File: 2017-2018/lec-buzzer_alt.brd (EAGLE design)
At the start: 160 x 100 mm, 26 parts, among them K1 SKQGADE010, K2 SKQGADE010, K3 SKQGADE010, U1 ATMEGA328P-MUR

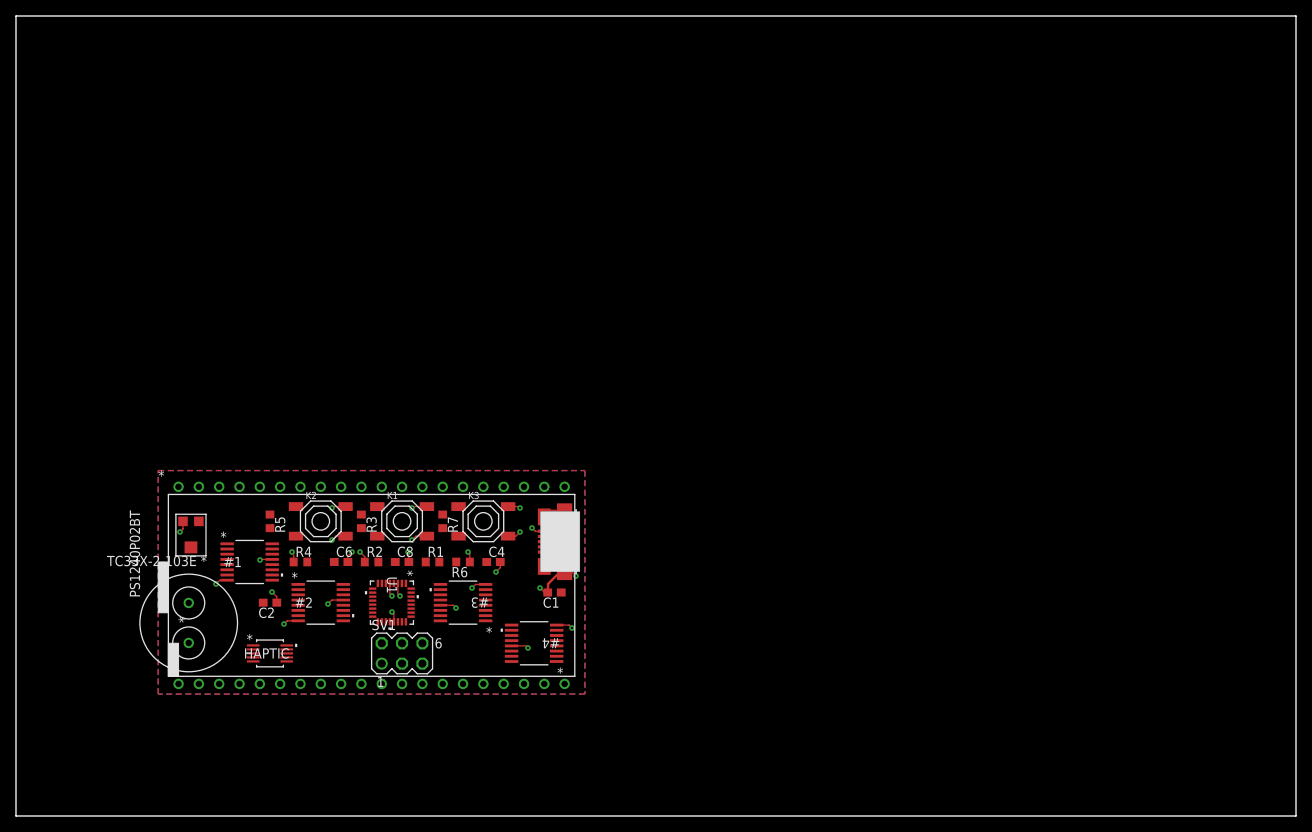
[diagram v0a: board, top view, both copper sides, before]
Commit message: 3 Button Board completed
LCD flipped, slight changes in shifter, Buzzer and SPI location
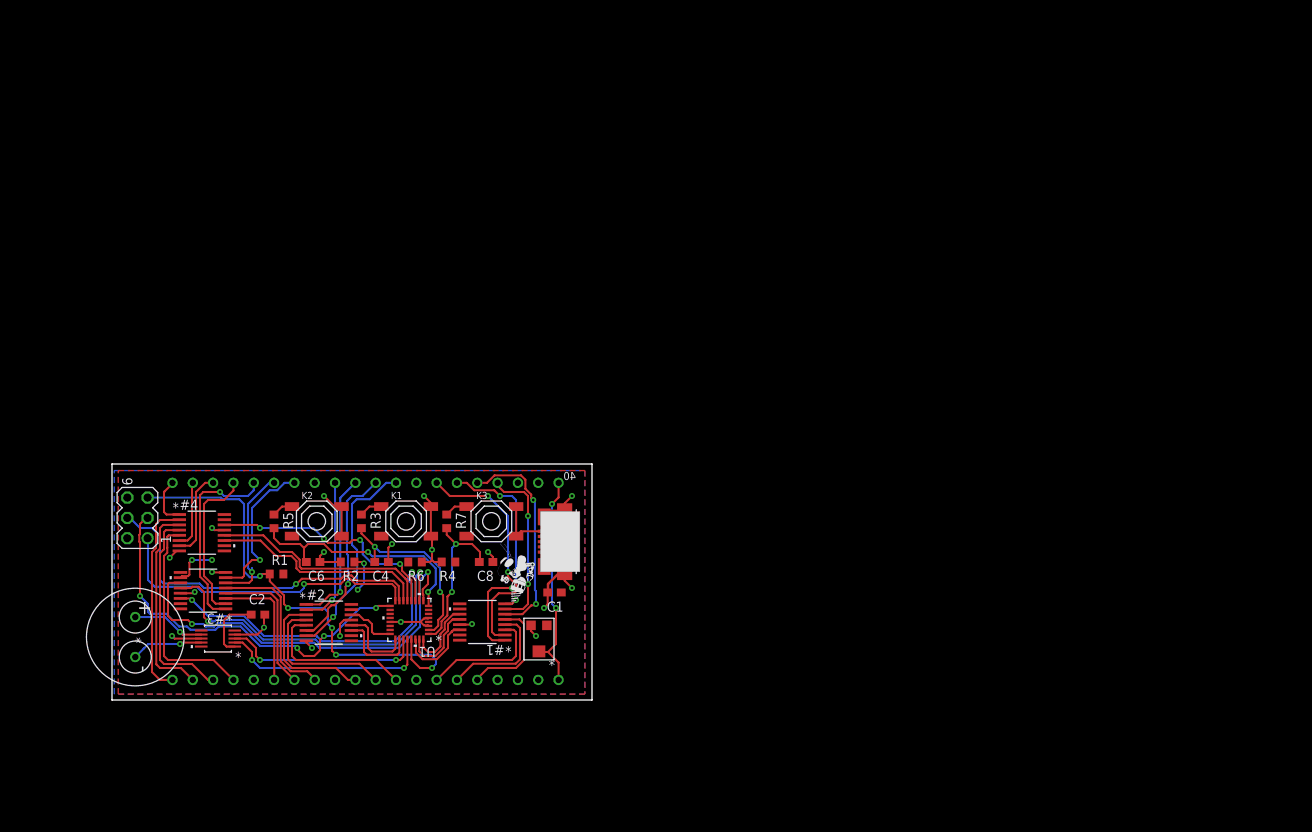
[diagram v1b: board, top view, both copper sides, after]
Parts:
- added U$2: (no value), RoboJackets-Aesthetics:ROBOBUZZ_0.4X
- moved LCD 47.5 mm to (67.8, 17.0), flipped to the bottom
- moved TC33X-2-103E 45.4 mm to (67.6, 25.1)
- moved #4 43.8 mm to (23.2, 35.4), turned to 0 degrees
- moved SV1 37.2 mm to (15.2, 37.3), turned to 90 degrees
- moved #3 32.5 mm to (23.4, 28.2)
- moved #1 30.0 mm to (58.3, 24.2), turned to 180 degrees
- moved R1 19.6 mm to (32.6, 30.2)
- moved R4 18.5 mm to (54.1, 31.8)
- moved C4 14.0 mm to (45.7, 31.8)
- moved C8 10.5 mm to (58.8, 31.8)
- moved PS1240P02BT 6.91 mm to (14.9, 22.4), turned to 270 degrees
- moved HAPTIC 6.76 mm to (25.2, 22.2), turned to 180 degrees
- moved R6 6.00 mm to (49.9, 31.8)
- moved C6 3.50 mm to (37.1, 31.8)
- moved U1 3.07 mm to (49.2, 24.5), turned to 180 degrees
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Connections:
- net !BTN2: now also U1.8; no longer U1.13
- net !BTN3: now also U1.1; no longer U1.14
- net SFT1: now also U1.30; no longer U1.10
- net SFT2: now also U1.24; no longer U1.7
- net SFT3: now also U1.11; no longer U1.25
- net SFT4: now also U1.12; no longer U1.1
- net SHIFT_CLK1: now also U1.31; no longer U1.11
- net SHIFT_CLK2: now also U1.25; no longer U1.8
- net SHIFT_CLK3: now also U1.10; no longer U1.30
- net SHIFT_CLK4: now also U1.13; no longer U1.32
- net STORAGE_CLK1: now also U1.32; no longer U1.12
- net STORAGE_CLK2: now also U1.26; no longer U1.9
- net STORAGE_CLK3: now also U1.9; no longer U1.26
- net STORAGE_CLK4: now also U1.14; no longer U1.31
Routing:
- net !RESET: track 0.00 -> 60.2 mm, vias 0 -> 5
- net STORAGE_CLK3: track 0.00 -> 51.5 mm, vias 0 -> 2
- net SCK: track 0.00 -> 49.1 mm, vias 0 -> 4
- net SHIFT_CLK3: track 0.00 -> 45.9 mm, vias 0 -> 2
- net MOSI: track 0.00 -> 43.8 mm, vias 0 -> 1
- net SFT3: track 0.00 -> 43.1 mm, vias 0 -> 2
- net MISO: track 0.00 -> 39.9 mm, vias 0 -> 1
- net 1A: track 0.00 -> 30.5 mm, vias 0 -> 2
- net !BTN2: track 0.00 -> 30.4 mm, vias 0 -> 2
- net SFT4: track 0.00 -> 30.3 mm, vias 0 -> 4
- net 1B: track 0.00 -> 29.8 mm, vias 0 -> 2
- net SHIFT_CLK4: track 0.00 -> 28.7 mm
- net DIVIDED: track 0.00 -> 27.3 mm, vias 0 -> 2
- net STORAGE_CLK4: track 0.00 -> 27.3 mm
- net 1F: track 0.00 -> 27.1 mm, vias 0 -> 2
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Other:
- board size 160 x 100 mm -> 60 x 29.5 mm
- board text added: "+"
- board text added: "-"
- board text added: "1"
- board text added: "20"
- board text added: "21"
- board text added: "40"
